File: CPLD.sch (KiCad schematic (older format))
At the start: 33 parts, among them J3 JTAG, SW2 User PB, SW3 User DIP, U2 74LVC1G04, U3 EPM7064STC100, X1 CFPS-72 50mhz

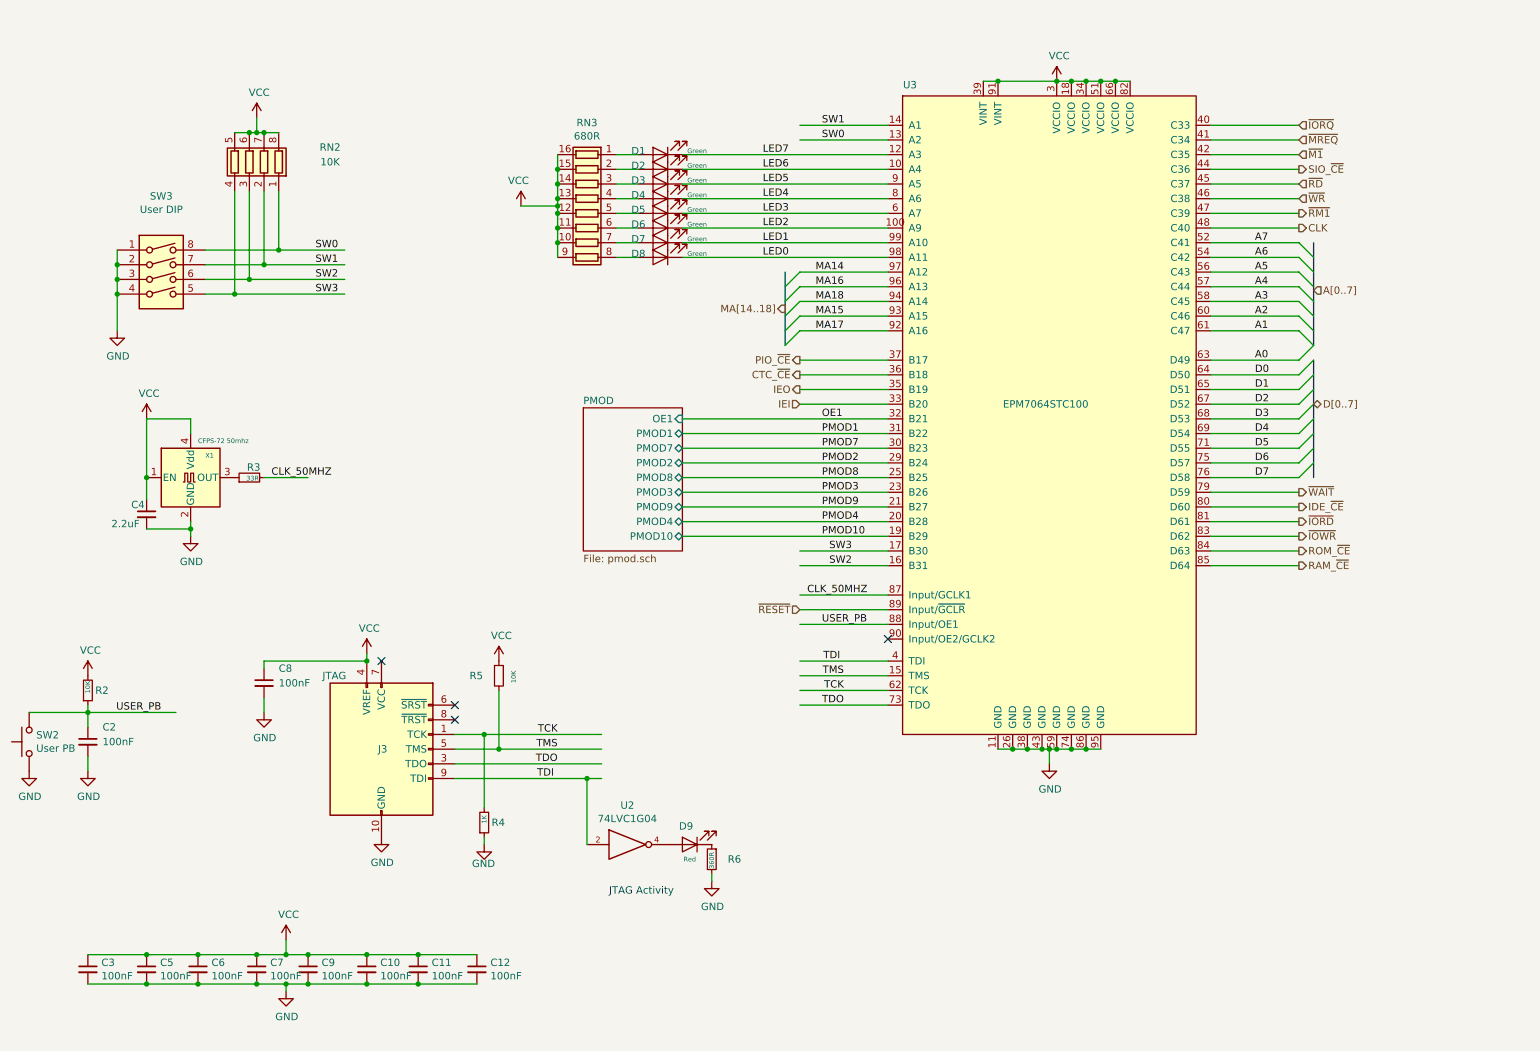
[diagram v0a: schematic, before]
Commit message: Routing finished
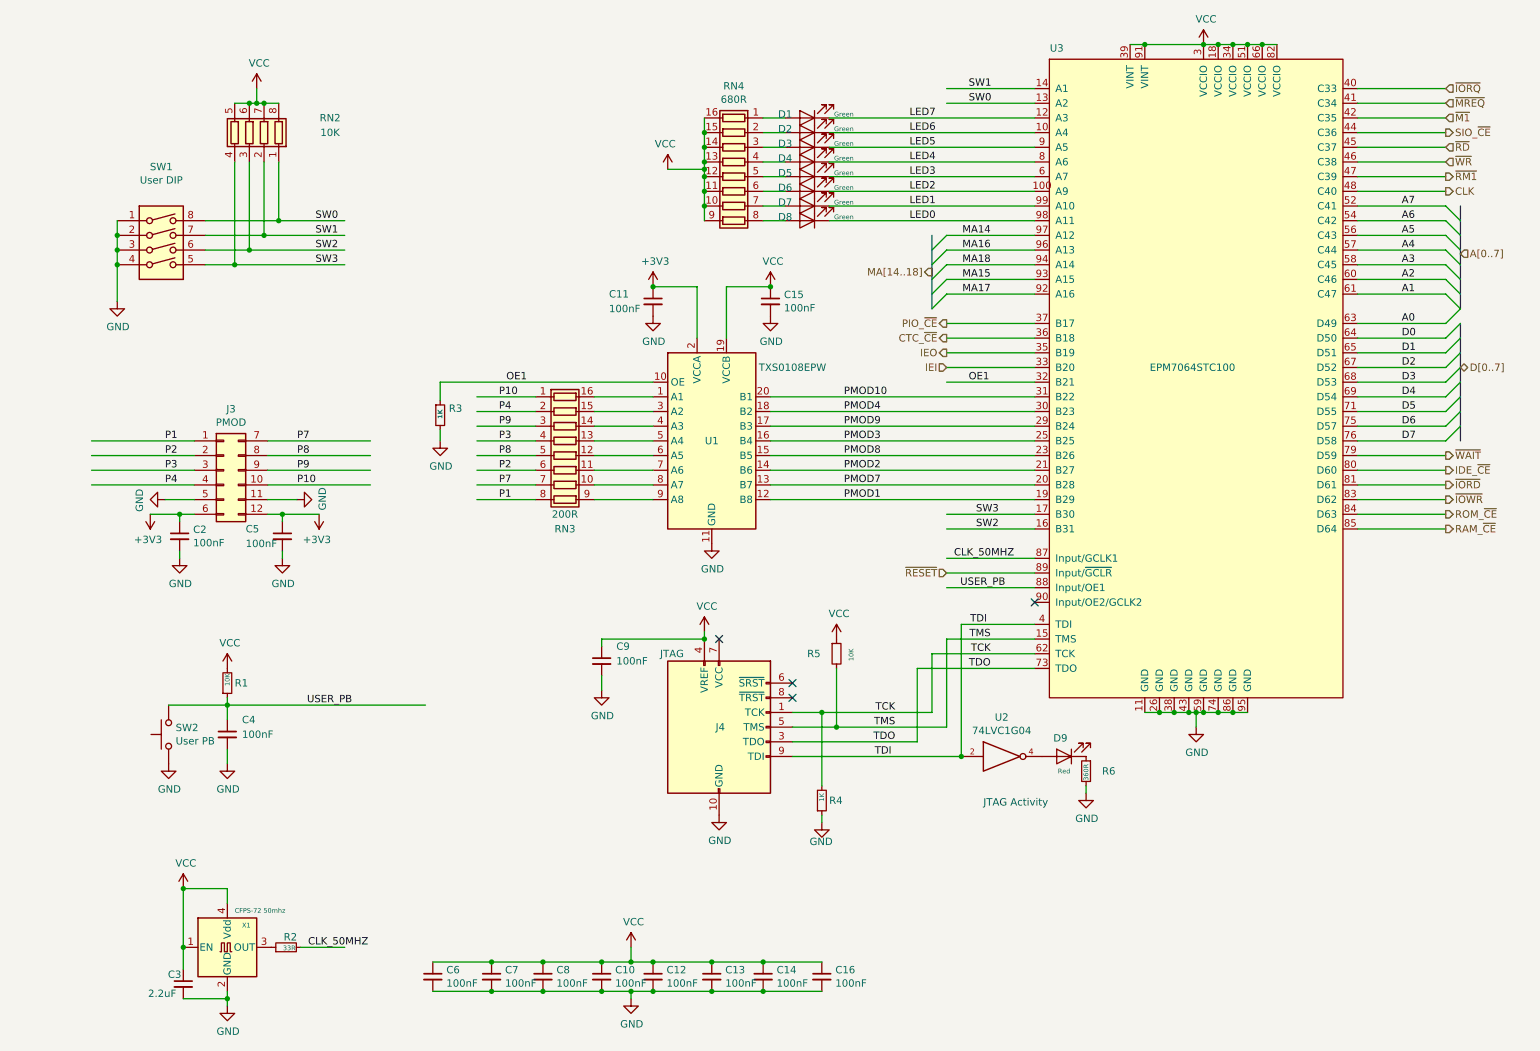
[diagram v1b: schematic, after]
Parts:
- added C11, C15, C2, C5: 100nF, Capacitor_SMD:C_0603_1608Metric_Pad1.05x0.95mm_HandSolder, symbol Device:C_Small
- added J3: PMOD, Connector_PinSocket_2.54mm:PinSocket_2x06_P2.54mm_Horizontal_Top_Bottom, symbol Connector_Generic:Conn_02x06_Top_Bottom
- added R3: 1K, Resistor_SMD:R_0603_1608Metric_Pad1.05x0.95mm_HandSolder, symbol Device:R_Small
- added RN3: 200R, Resistor_SMD:R_Cat16-8, symbol Device:R_Pack08
- added U1: TXS0108EPW, Package_SO:TSSOP-20_4.4x6.5mm_P0.65mm, symbol Logic_LevelTranslator:TXS0108EPW
- renumbered C7 to C10, C9 to C12, C10 to C13, C11 to C14, C12 to C16, C4 to C3, C2 to C4, C3 to C6, C5 to C7, C6 to C8, C8 to C9, J3 to J4, R2 to R1, R3 to R2, RN3 to RN4, SW3 to SW1
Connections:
- net labels added: +3V3, P1, P10, P2, P3, P4, P7, P8, P9
- wire segments 168 -> 211
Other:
- moved on the sheet: C10, C12, C13, C14, C16, C3, C4, C6, C7, C8, C9, D1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
